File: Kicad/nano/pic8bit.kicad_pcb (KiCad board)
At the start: 2 copper layers, 21 x 52 mm, 38 parts, among them K1 MCU 1, K2 MCU 2, K3 ICSP, K4 POWER & UART, U1 PIC16F/PIC18F, U2 MCP2221A-IST, U3 BU33SD5WG

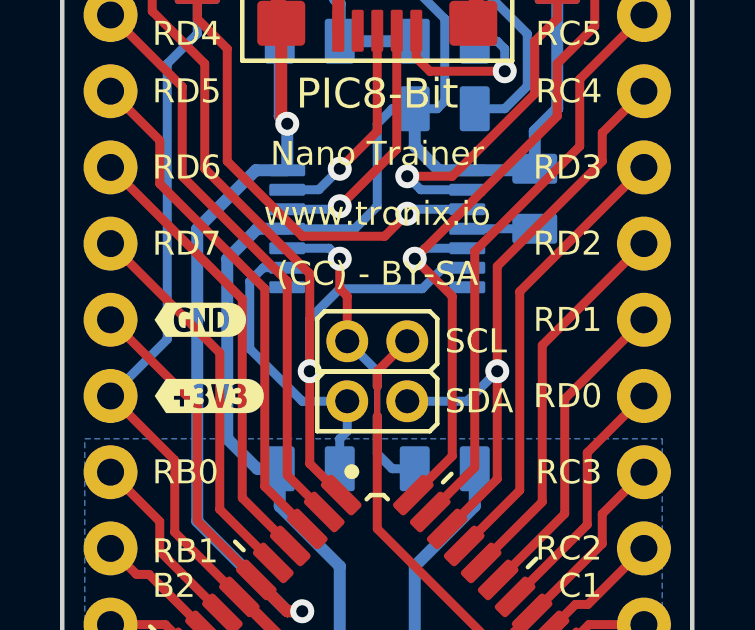
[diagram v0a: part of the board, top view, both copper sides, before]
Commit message: Update Nano
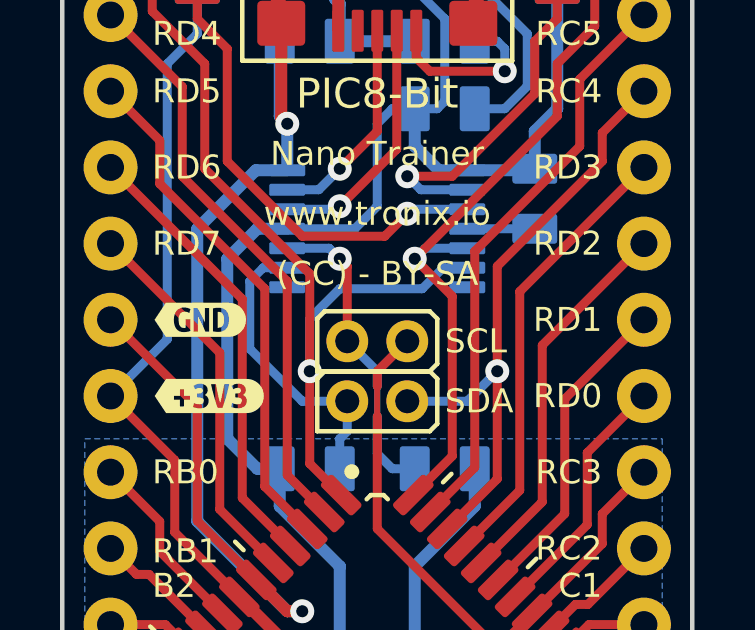
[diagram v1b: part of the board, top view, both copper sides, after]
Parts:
- R1: value 4K7 -> 10K
- U2: value MCP2221A-IST -> MCP2221A
